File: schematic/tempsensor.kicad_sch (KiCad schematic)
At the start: 6 parts

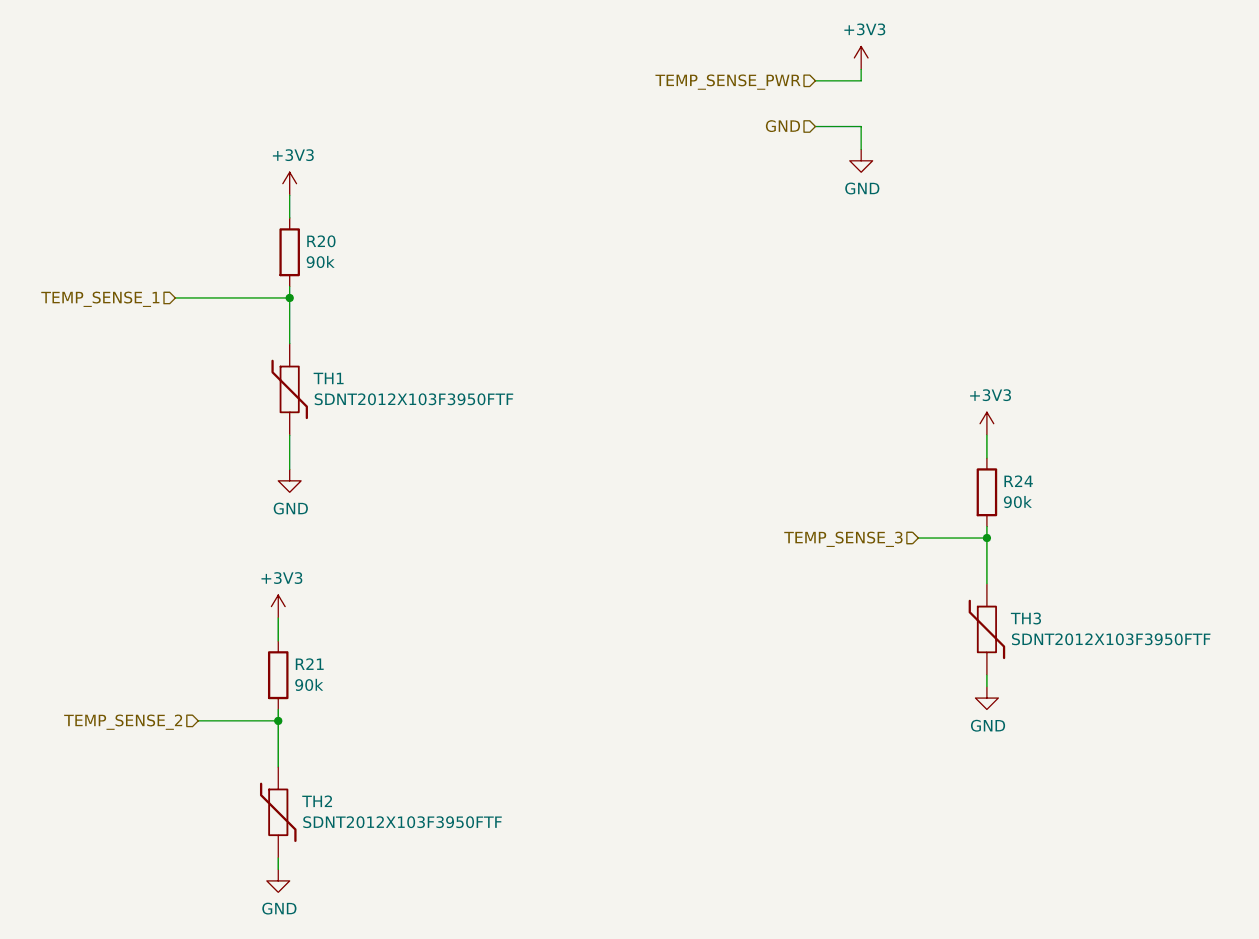
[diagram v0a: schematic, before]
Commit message: d
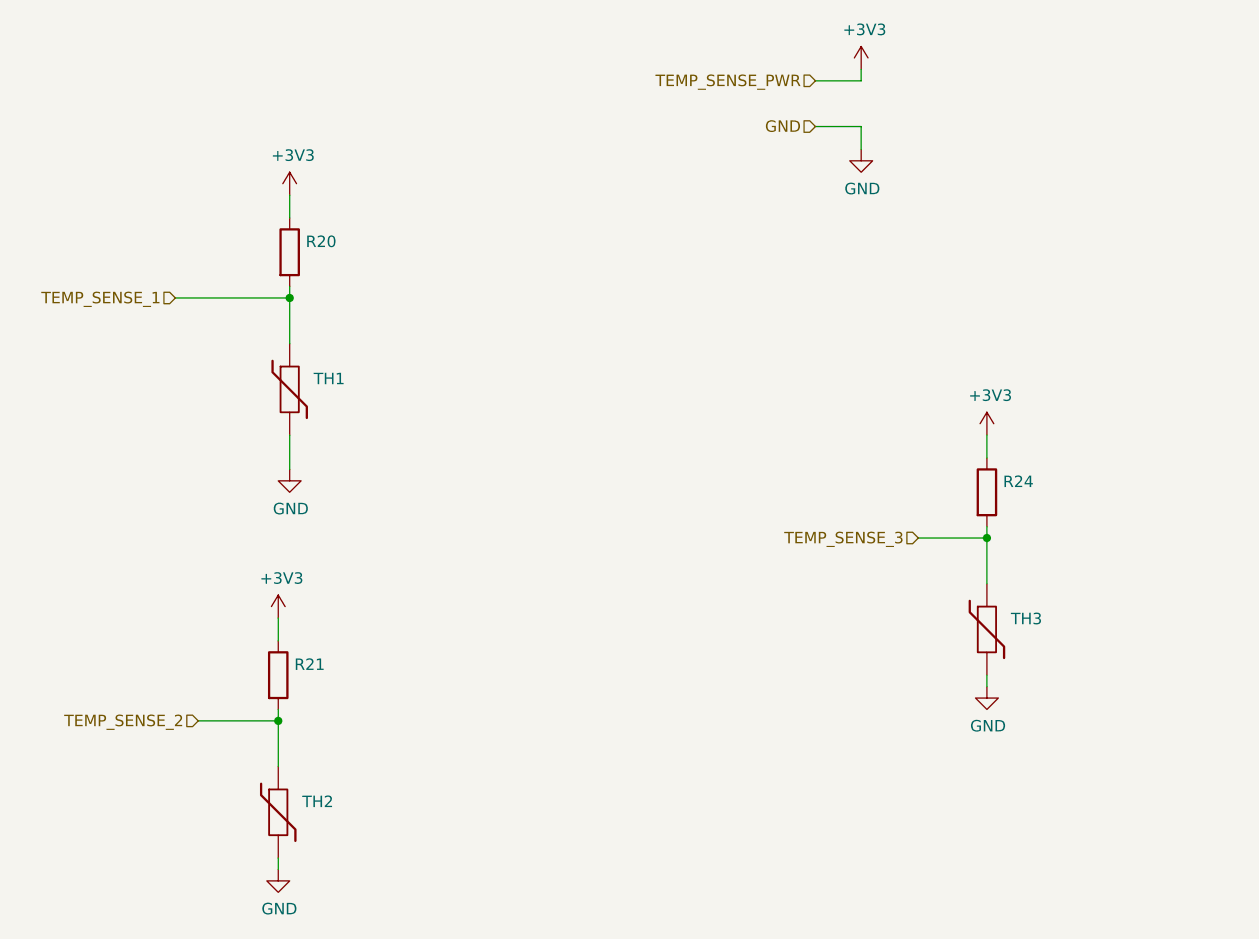
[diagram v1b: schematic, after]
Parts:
- R20, R21, R24: value 90k -> (none); footprint Resistor_SMD:R_0805_2012Metric_Pad1.20x1.40mm_HandSolder -> (none)
- TH1, TH2, TH3: value SDNT2012X103F3950FTF -> (none); footprint Resistor_SMD:R_0805_2012Metric_Pad1.20x1.40mm_HandSolder -> (none)
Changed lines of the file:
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@@
       (effects (font (size 1.27 1.27)) (justify left))
     )
-    (property "Value" "SDNT2012X103F3950FTF" (id 1) (at 123.317 79.883 0)
+    (property "Value" "" (id 1) (at 123.317 79.883 0)
       (effects (font (size 1.27 1.27)) (justify left))
     )
-    (property "Footprint" "Resistor_SMD:R_0805_2012Metric_Pad1.20x1.40mm_HandSolder" (id 2) (at 120.65 78.74 0)
+    (property "Footprint" "" (id 2) (at 120.65 78.74 0)
       (effects (font (size 1.27 1.27)) hide)
     )
@@
       (effects (font (size 1.27 1.27)) (justify left))
     )
-    (property "Value" "90k" (id 1) (at 122.428 64.643 0)
+    (property "Value" "" (id 1) (at 122.428 64.643 0)
       (effects (font (size 1.27 1.27)) (justify left))
     )
-    (property "Footprint" "Resistor_SMD:R_0805_2012Metric_Pad1.20x1.40mm_HandSolder" (id 2) (at 118.872 63.5 90)
+    (property "Footprint" "" (id 2) (at 118.872 63.5 90)
       (effects (font (size 1.27 1.27)) hide)
     )
@@
       (effects (font (size 1.27 1.27)) (justify left))
     )
-    (property "Value" "SDNT2012X103F3950FTF" (id 1) (at 122.047 126.873 0)
+    (property "Value" "" (id 1) (at 122.047 126.873 0)
       (effects (font (size 1.27 1.27)) (justify left))
     )
-    (property "Footprint" "Resistor_SMD:R_0805_2012Metric_Pad1.20x1.40mm_HandSolder" (id 2) (at 119.38 125.73 0)
+    (property "Footprint" "" (id 2) (at 119.38 125.73 0)
       (effects (font (size 1.27 1.27)) hide)
     )
@@
       (effects (font (size 1.27 1.27)) (justify left))
     )
-    (property "Value" "90k" (id 1) (at 121.158 111.633 0)
+    (property "Value" "" (id 1) (at 121.158 111.633 0)
       (effects (font (size 1.27 1.27)) (justify left))
     )
-    (property "Footprint" "Resistor_SMD:R_0805_2012Metric_Pad1.20x1.40mm_HandSolder" (id 2) (at 117.602 110.49 90)
+    (property "Footprint" "" (id 2) (at 117.602 110.49 90)
       (effects (font (size 1.27 1.27)) hide)
     )
@@
       (effects (font (size 1.27 1.27)) (justify left))
     )
-    (property "Value" "SDNT2012X103F3950FTF" (id 1) (at 200.787 106.553 0)
+    (property "Value" "" (id 1) (at 200.787 106.553 0)
       (effects (font (size 1.27 1.27)) (justify left))
     )
-    (property "Footprint" "Resistor_SMD:R_0805_2012Metric_Pad1.20x1.40mm_HandSolder" (id 2) (at 198.12 105.41 0)
+    (property "Footprint" "" (id 2) (at 198.12 105.41 0)
       (effects (font (size 1.27 1.27)) hide)
     )
@@
       (effects (font (size 1.27 1.27)) (justify left))
     )
-    (property "Value" "90k" (id 1) (at 199.898 91.313 0)
+    (property "Value" "" (id 1) (at 199.898 91.313 0)
       (effects (font (size 1.27 1.27)) (justify left))
     )
-    (property "Footprint" "Resistor_SMD:R_0805_2012Metric_Pad1.20x1.40mm_HandSolder" (id 2) (at 196.342 90.17 90)
+    (property "Footprint" "" (id 2) (at 196.342 90.17 90)
       (effects (font (size 1.27 1.27)) hide)
     )

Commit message: e
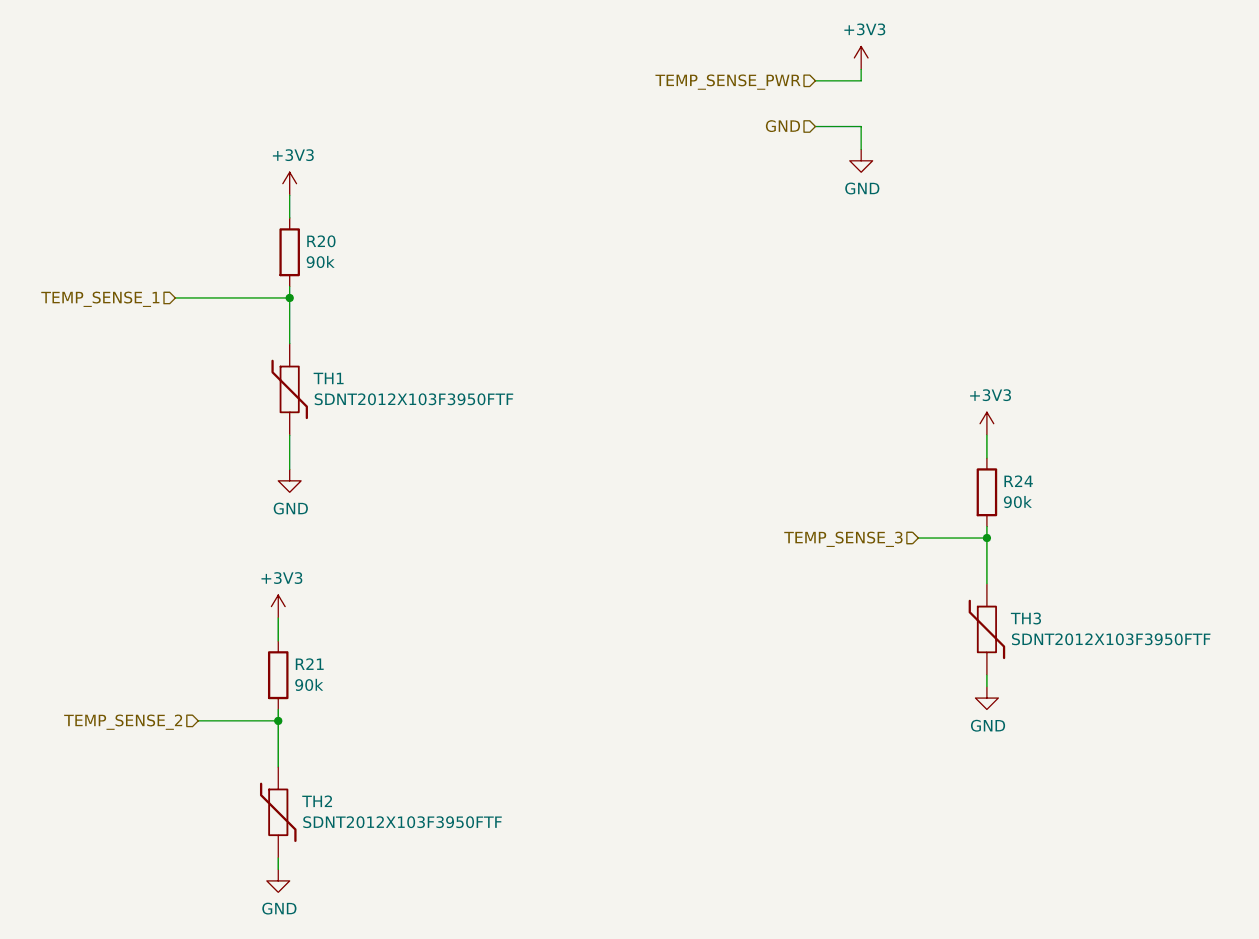
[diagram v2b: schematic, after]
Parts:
- R20, R21, R24: value (none) -> 90k; footprint (none) -> Resistor_SMD:R_0805_2012Metric_Pad1.20x1.40mm_HandSolder
- TH1, TH2, TH3: value (none) -> SDNT2012X103F3950FTF; footprint (none) -> Resistor_SMD:R_0805_2012Metric_Pad1.20x1.40mm_HandSolder
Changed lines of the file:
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@@
       (effects (font (size 1.27 1.27)) (justify left))
     )
-    (property "Value" "" (id 1) (at 123.317 79.883 0)
+    (property "Value" "SDNT2012X103F3950FTF" (id 1) (at 123.317 79.883 0)
       (effects (font (size 1.27 1.27)) (justify left))
     )
-    (property "Footprint" "" (id 2) (at 120.65 78.74 0)
+    (property "Footprint" "Resistor_SMD:R_0805_2012Metric_Pad1.20x1.40mm_HandSolder" (id 2) (at 120.65 78.74 0)
       (effects (font (size 1.27 1.27)) hide)
     )
@@
       (effects (font (size 1.27 1.27)) (justify left))
     )
-    (property "Value" "" (id 1) (at 122.428 64.643 0)
+    (property "Value" "90k" (id 1) (at 122.428 64.643 0)
       (effects (font (size 1.27 1.27)) (justify left))
     )
-    (property "Footprint" "" (id 2) (at 118.872 63.5 90)
+    (property "Footprint" "Resistor_SMD:R_0805_2012Metric_Pad1.20x1.40mm_HandSolder" (id 2) (at 118.872 63.5 90)
       (effects (font (size 1.27 1.27)) hide)
     )
@@
       (effects (font (size 1.27 1.27)) (justify left))
     )
-    (property "Value" "" (id 1) (at 122.047 126.873 0)
+    (property "Value" "SDNT2012X103F3950FTF" (id 1) (at 122.047 126.873 0)
       (effects (font (size 1.27 1.27)) (justify left))
     )
-    (property "Footprint" "" (id 2) (at 119.38 125.73 0)
+    (property "Footprint" "Resistor_SMD:R_0805_2012Metric_Pad1.20x1.40mm_HandSolder" (id 2) (at 119.38 125.73 0)
       (effects (font (size 1.27 1.27)) hide)
     )
@@
       (effects (font (size 1.27 1.27)) (justify left))
     )
-    (property "Value" "" (id 1) (at 121.158 111.633 0)
+    (property "Value" "90k" (id 1) (at 121.158 111.633 0)
       (effects (font (size 1.27 1.27)) (justify left))
     )
-    (property "Footprint" "" (id 2) (at 117.602 110.49 90)
+    (property "Footprint" "Resistor_SMD:R_0805_2012Metric_Pad1.20x1.40mm_HandSolder" (id 2) (at 117.602 110.49 90)
       (effects (font (size 1.27 1.27)) hide)
     )
@@
       (effects (font (size 1.27 1.27)) (justify left))
     )
-    (property "Value" "" (id 1) (at 200.787 106.553 0)
+    (property "Value" "SDNT2012X103F3950FTF" (id 1) (at 200.787 106.553 0)
       (effects (font (size 1.27 1.27)) (justify left))
     )
-    (property "Footprint" "" (id 2) (at 198.12 105.41 0)
+    (property "Footprint" "Resistor_SMD:R_0805_2012Metric_Pad1.20x1.40mm_HandSolder" (id 2) (at 198.12 105.41 0)
       (effects (font (size 1.27 1.27)) hide)
     )
@@
       (effects (font (size 1.27 1.27)) (justify left))
     )
-    (property "Value" "" (id 1) (at 199.898 91.313 0)
+    (property "Value" "90k" (id 1) (at 199.898 91.313 0)
       (effects (font (size 1.27 1.27)) (justify left))
     )
-    (property "Footprint" "" (id 2) (at 196.342 90.17 90)
+    (property "Footprint" "Resistor_SMD:R_0805_2012Metric_Pad1.20x1.40mm_HandSolder" (id 2) (at 196.342 90.17 90)
       (effects (font (size 1.27 1.27)) hide)
     )
